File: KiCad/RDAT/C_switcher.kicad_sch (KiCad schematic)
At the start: 12 parts, among them J3 USB_C_Receptacle, U5 SN2002011RSHR

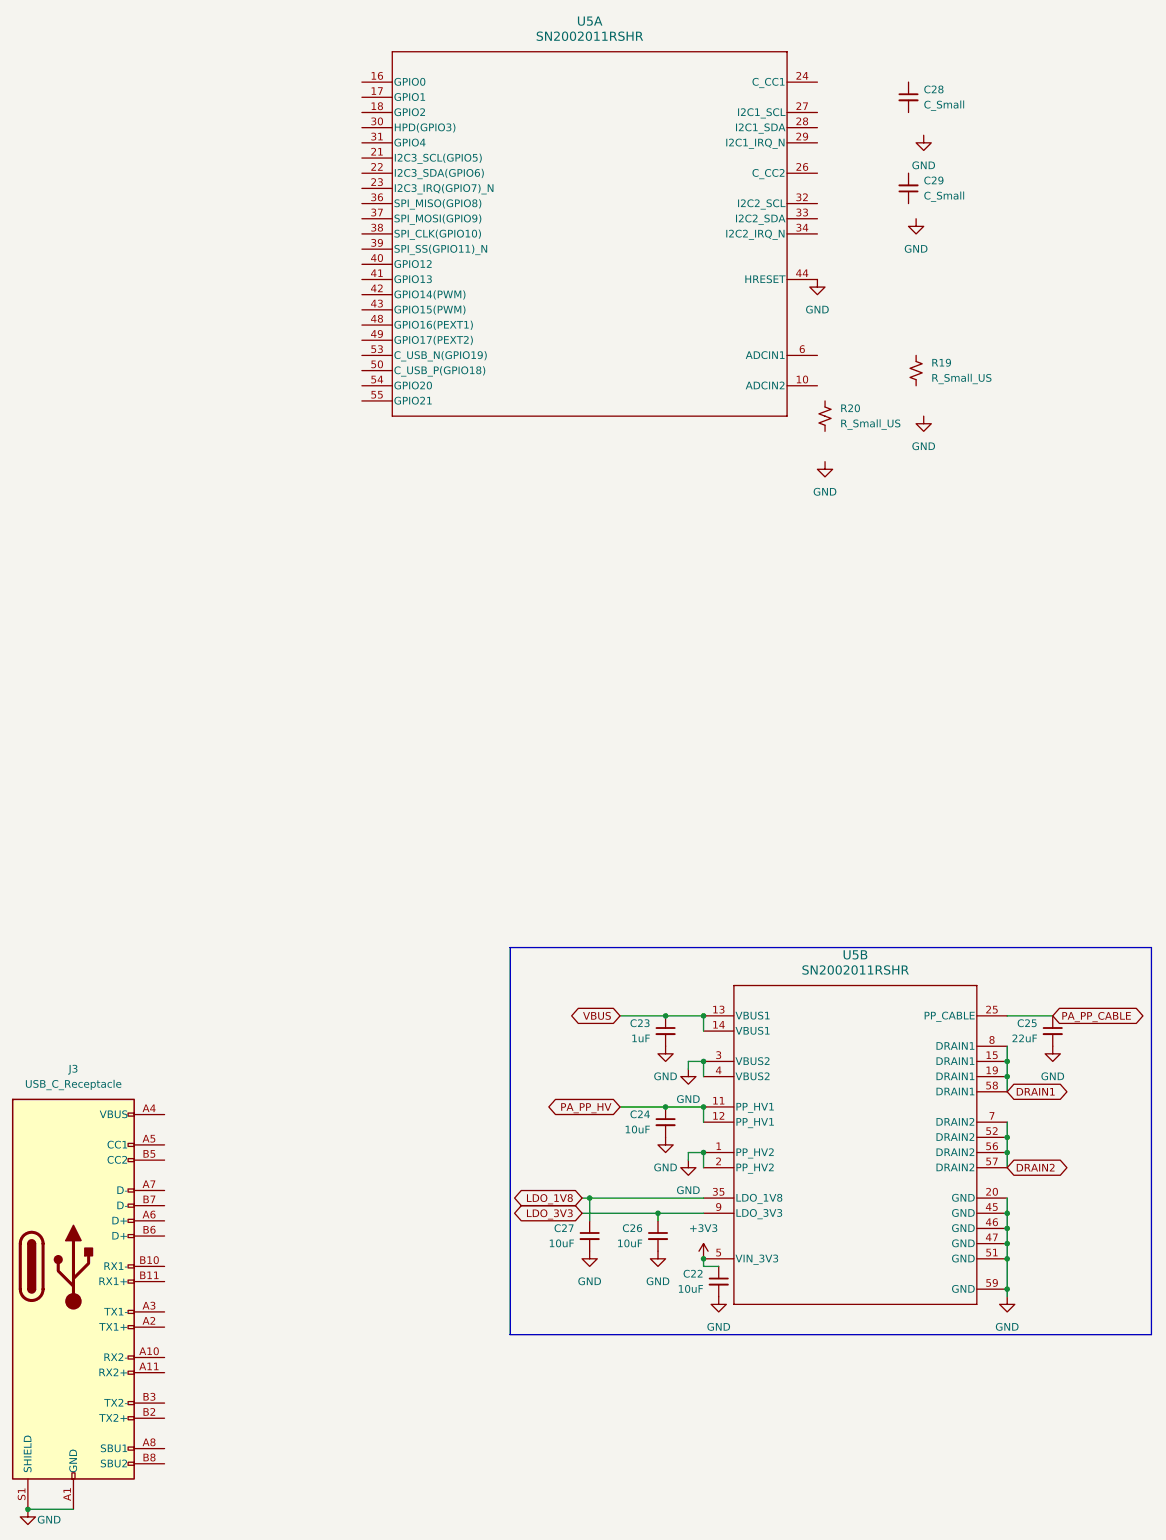
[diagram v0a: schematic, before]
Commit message: Update BMS
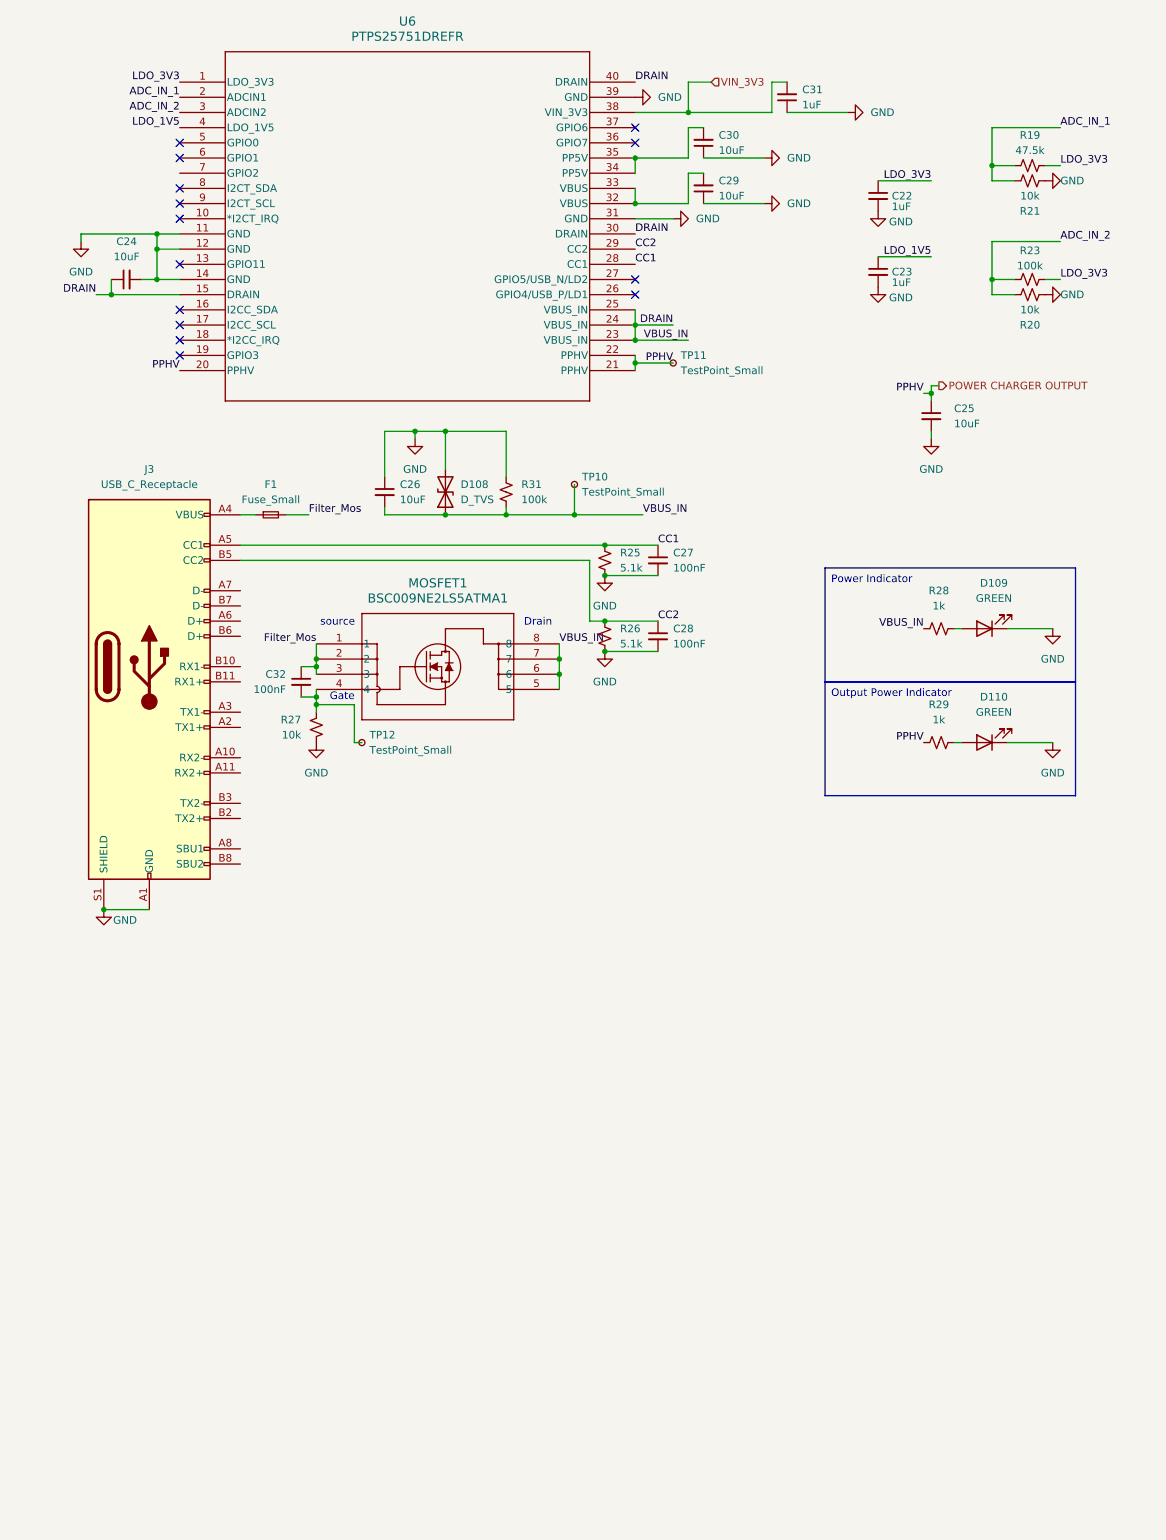
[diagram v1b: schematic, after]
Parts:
- removed U5: SN2002011RSHR, RSH0056E-MFG, symbol TPS65987DDK:SN2002011RSHR
- added C30: 10uF, symbol Device:C_Small
- added C31: 1uF, symbol Device:C_Small
- added C32: 100nF, symbol Device:C_Small
- added D108: D_TVS, symbol Device:D_TVS
- added D109, D110: GREEN, symbol Device:LED
- added F1: Fuse_Small, symbol Device:Fuse_Small
- added MOSFET1: BSC009NE2LS5ATMA1, PG-TDSON-8-1_INF, symbol BSC009NE2LS5ATMA1:BSC009NE2LS5ATMA1
- added R21, R27: 10k, symbol Device:R_Small_US
- added R23, R31: 100k, symbol Device:R_Small_US
- added R25, R26: 5.1k, symbol Device:R_Small_US
- added R28, R29: 1k, symbol Device:R_Small_US
- added TP10, TP11, TP12: TestPoint_Small, symbol Connector:TestPoint_Small
- added U6: PTPS25751DREFR, WQFN38_REF_TEX, symbol TPS25751:PTPS25751DREFR
- C22: value 10uF -> 1uF
- C25: value 22uF -> 10uF
- C27: value 10uF -> 100nF
- C28: value C_Small -> 100nF
- C29: value C_Small -> 10uF
- R19: value R_Small_US -> 47.5k
- R20: value R_Small_US -> 10k
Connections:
- net +3V3 is gone; now on net LDO_3V3: C22.1
- net LDO_1V8 is gone; now on net CC1: C27.1
- net GND: now also C26.1, C28.2, C29.1, R20.1, C30.1, C31.1, D108.2 (A2), D109.1 (K), D110.1 (K), R21.1, R25.2, R26.2, R27.2, R31.1, U6.11 (GND), U6.12 (GND), U6.14 (GND), U6.31 (GND), U6.39 (GND); no longer C26.2
- net LDO_3V3: now also R19.2, R23.2, U6.1 (LDO_3V3); no longer C26.1
- net at J3.A4 (VBUS), J3.A9 (VBUS), J3.B4 (VBUS)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: now also F1.1
- net CC1: now reaches J3.A5 (CC1)
- net CC1: now also R25.1, U6.28 (CC1)
- net CC2: now reaches J3.B5 (CC2)
- net CC2: now also C28.1, R26.1, U6.29 (CC2)
- net ADC_IN_1: now reaches R19.1
- net ADC_IN_1: now also R21.2, U6.2 (ADCIN1)
- net ADC_IN_2: now reaches R20.2
- net ADC_IN_2: now also R23.1, U6.3 (ADCIN2)
- net at C29.2: now also U6.32 (VBUS), U6.33 (VBUS)
- net PA_PP_CABLE renamed POWER CHARGER OUTPUT
- net POWER CHARGER OUTPUT: now also R29.2, TP11.1, U6.20 (PPHV), U6.21 (PPHV), U6.22 (PPHV)
- net PA_PP_HV renamed DRAIN
- net DRAIN: now also C26.2, D108.1 (A1), MOSFET1.5, MOSFET1.6, MOSFET1.7, MOSFET1.8, R28.2, R31.2, TP10.1, U6.15 (DRAIN), U6.23 (VBUS_IN), U6.24 (VBUS_IN), U6.25 (VBUS_IN), U6.30 (DRAIN), U6.40 (DRAIN)
- net VBUS renamed LDO_1V5
- net LDO_1V5: now also U6.4 (LDO_1V5)
- new net: C32.2, MOSFET1.4, R27.1, TP12.1
- new net: D109.2 (A), R28.1
- new net: D110.2 (A), R29.1
- new net: C30.2, U6.34 (PP5V), U6.35 (PP5V)
- new net Filter_Mos: C32.1, F1.2, MOSFET1.1, MOSFET1.2, MOSFET1.3
- new net VIN_3V3: C31.2, U6.38 (VIN_3V3)
- no-connect marks 0 -> 14
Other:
- note added: "Drain"
- note added: "Gate"
- note added: "source"
